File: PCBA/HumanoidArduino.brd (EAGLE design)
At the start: 105.4 x 75.2 mm, 76 parts, among them IC1 7805TV, J2 22-27-2041-04

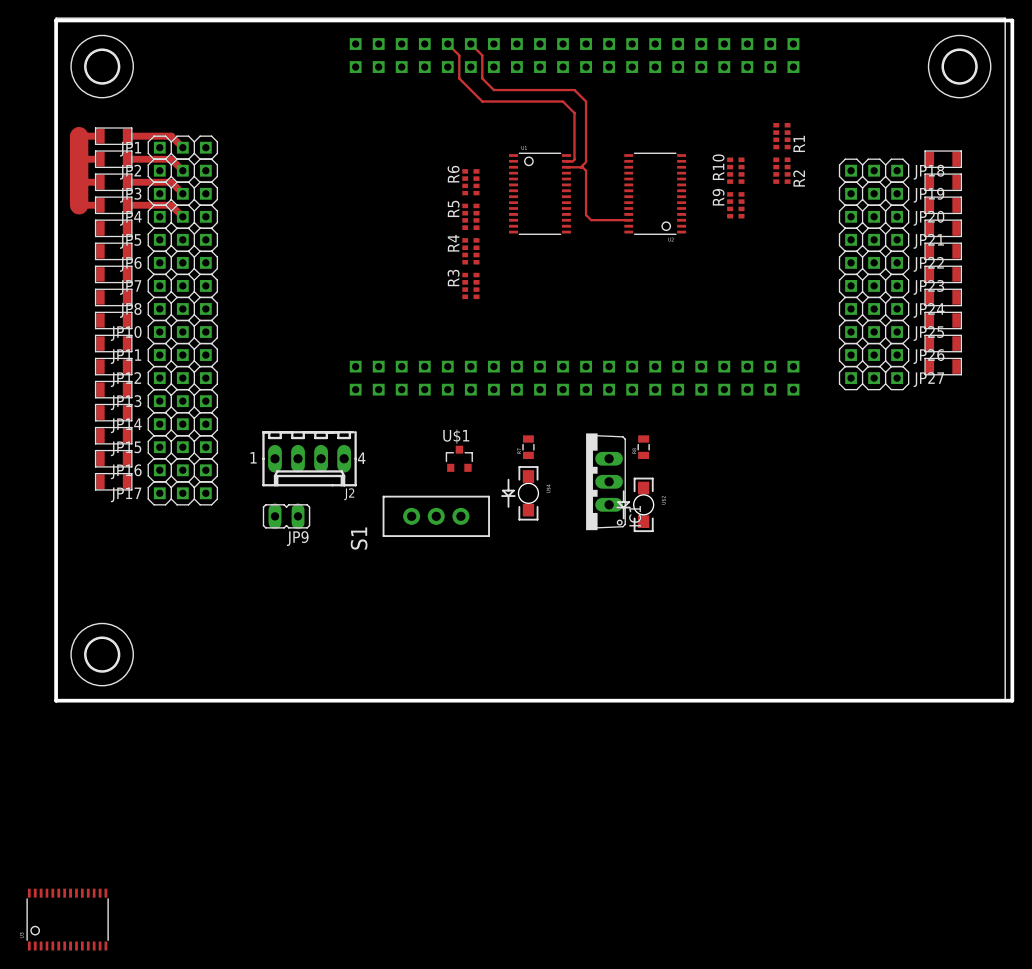
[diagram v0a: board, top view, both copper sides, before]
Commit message: Working on PCB
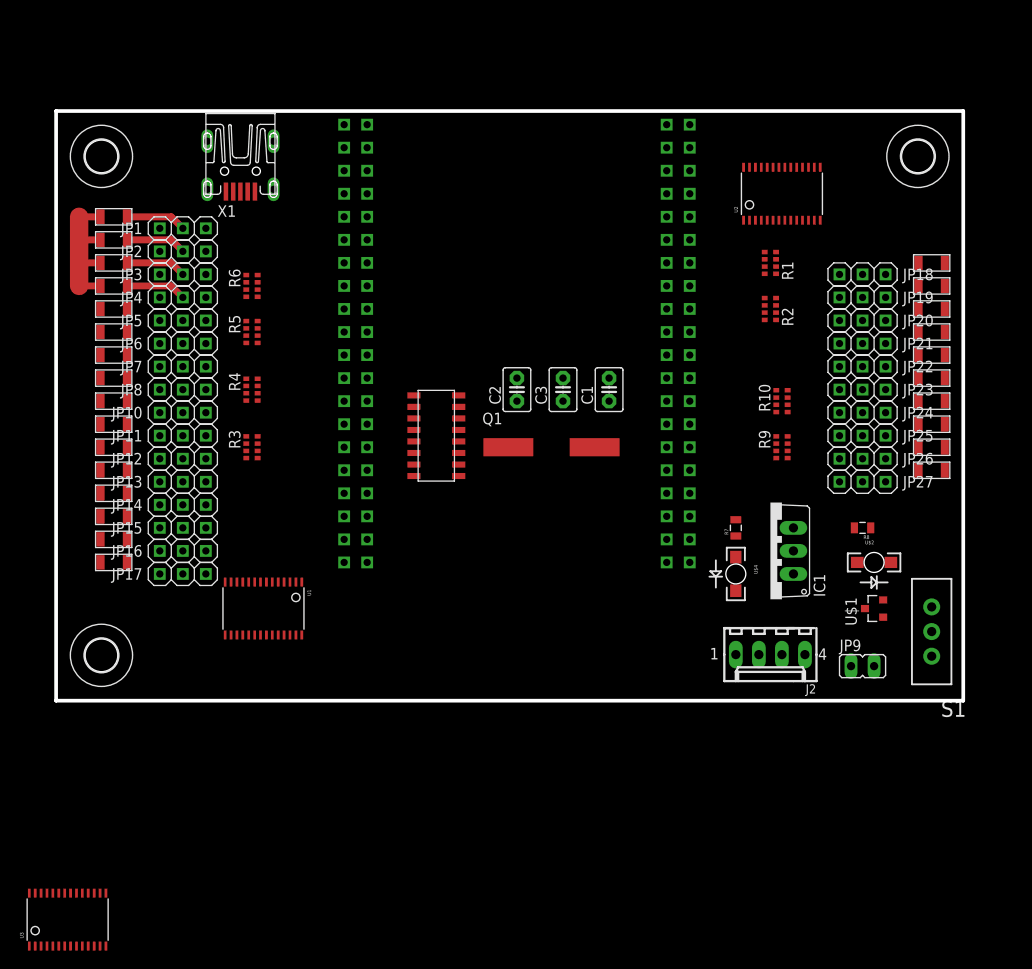
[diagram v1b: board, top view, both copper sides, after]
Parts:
- added C1: 100nF, capacitor-wima:C2.5-3
- added C2, C3: 22p, capacitor-wima:C2.5-3
- added Q1: 12MHz, crystal:CSM-7X-DU
- added U4: CH340G, HumanoidLbr:SO-16
- added X1: MINI-USB-UX60-MB-5S8, con-hirose:UX60-MB-5S8
- moved JP9 65.6 mm to (88.9, 3.81), turned to 270 degrees
- moved S1 56.1 mm to (96.5, 7.62), turned to 180 degrees
- moved J2 55.2 mm to (78.7, 5.08)
- moved U1 54.9 mm to (22.9, 10.2), turned to 180 degrees
- moved U$3 50.3 mm to (31.8, 63.5), turned to 180 degrees
- moved U$1 48.6 mm to (90.2, 10.2), turned to 90 degrees
- moved R3 30.0 mm to (21.6, 27.9)
- moved R4 28.5 mm to (21.6, 34.3)
- moved R5 27.3 mm to (21.6, 40.6)
- moved R9 27.1 mm to (80.0, 27.9)
- moved R6 26.7 mm to (21.6, 45.7)
- moved U$2 26.2 mm to (90.2, 15.2), turned to 0 degrees
- moved R10 25.9 mm to (80.0, 33.0)
- moved R8 25.7 mm to (88.9, 19.1), turned to 180 degrees
- moved R7 24.5 mm to (74.9, 19.1)
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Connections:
- new net D+: U4.5, X1.3
- new net D-: U4.6, X1.2
- new net N$56: C2.1, Q1.2, U4.7
- new net N$57: C3.1, Q1.1, U4.8
- new net RX: U$3.UART1-TX, U4.3
- new net TX: U$3.UART1-RX, U4.2
- net +5V: now also C1.1, U4.16, X1.1
- net GND: now also C1.2, C2.2, C3.2, U4.1, X1.5
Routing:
- net SCL: track 36.4 -> 0.00 mm
- net SDA: track 24.7 -> 0.00 mm
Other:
- board size 105.4 x 75.2 mm -> 100 x 65 mm
